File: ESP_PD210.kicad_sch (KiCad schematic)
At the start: 68 parts, among them J1 TTL, J2 CART, J3 USB_C_Receptacle_USB2.0, Q1 NPN, Q2 SE30P09D, SW1 Rocker, SW2 Move, U1 SSD1316, U2 ESP8684, U3 OPA188, U4 JW5017S, U5 CH221K, X1 SG-211

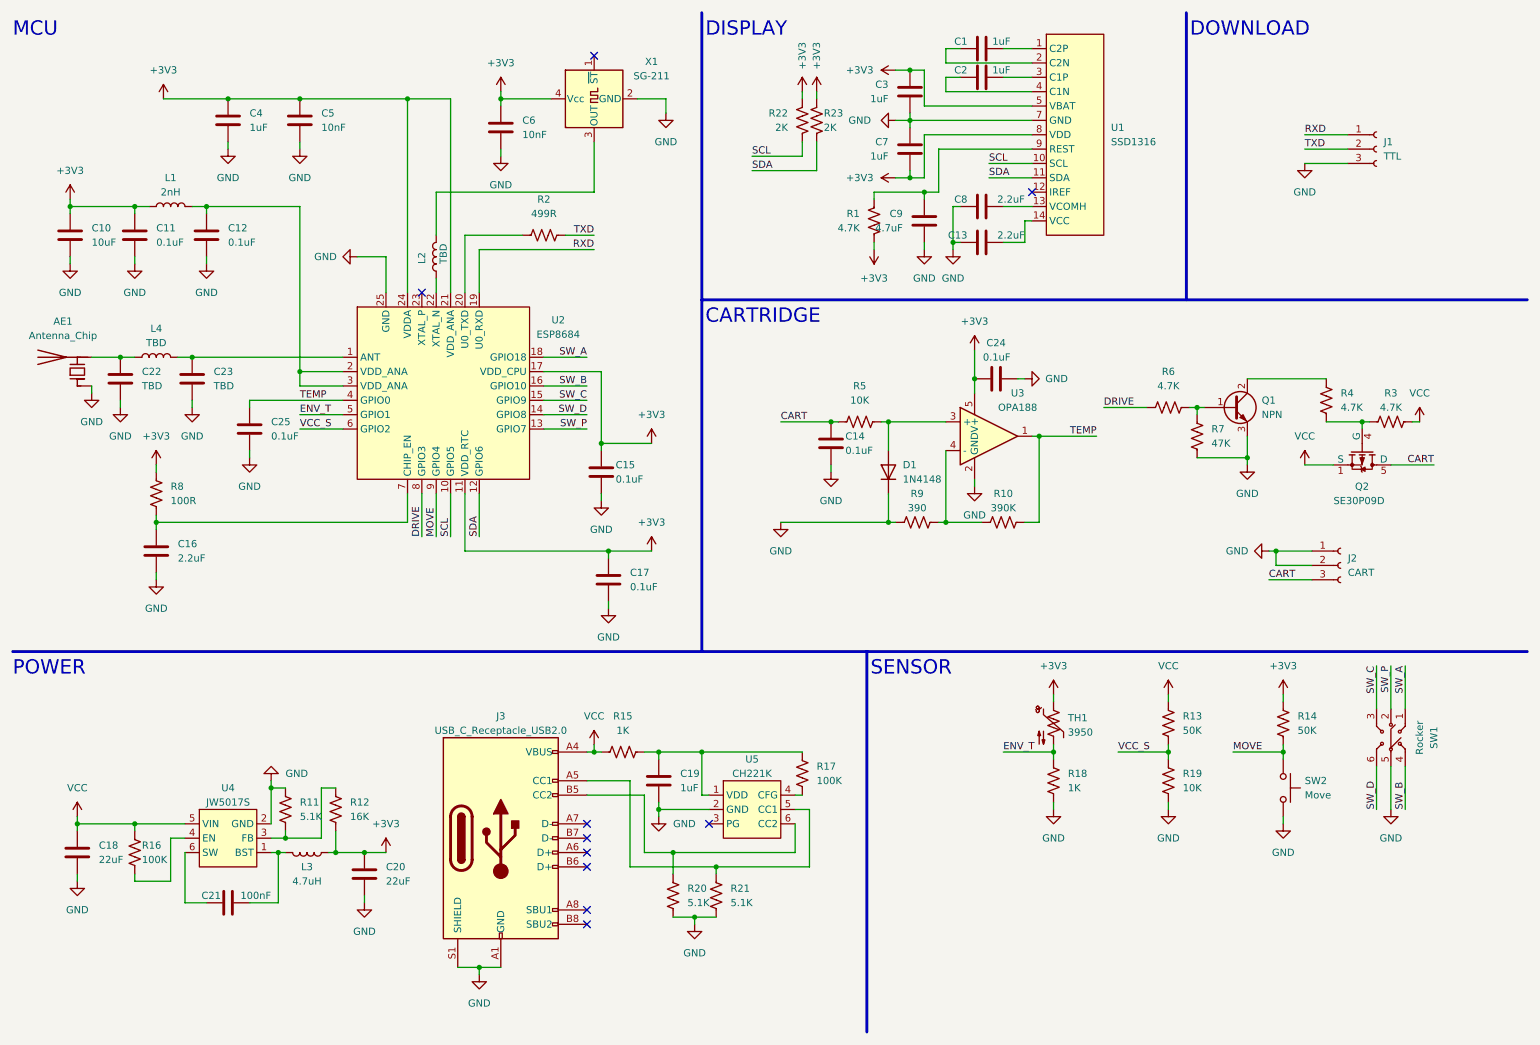
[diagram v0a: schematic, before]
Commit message: Optimize the layout
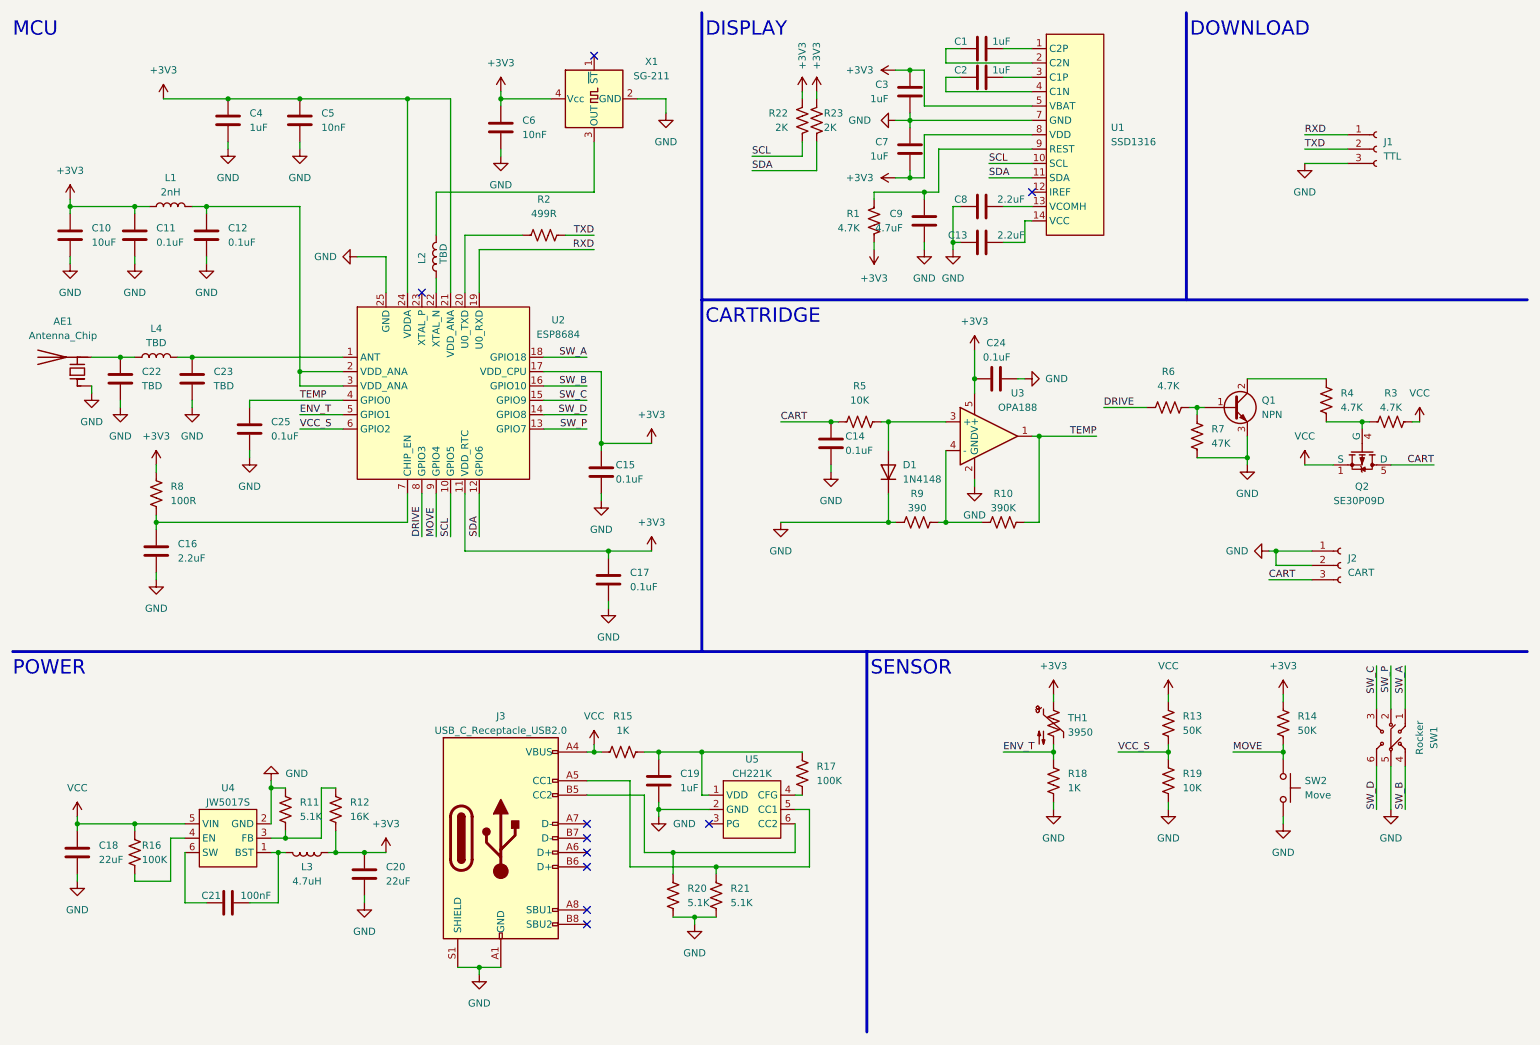
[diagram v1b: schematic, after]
